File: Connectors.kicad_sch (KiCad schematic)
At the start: 12 parts, among them J10 Conn_01x12_MountingPin, J11 Conn_01x09, J15 Conn_01x12_MountingPin, J19 Conn_01x12_MountingPin, J20 Conn_01x12_MountingPin, J21 Conn_01x12_MountingPin, J25 Conn_01x03, J26 Conn_01x04, J27 Conn_01x02, J5 Conn_01x12_MountingPin, J6 Conn_01x12_MountingPin, J8 Conn_01x12_MountingPin

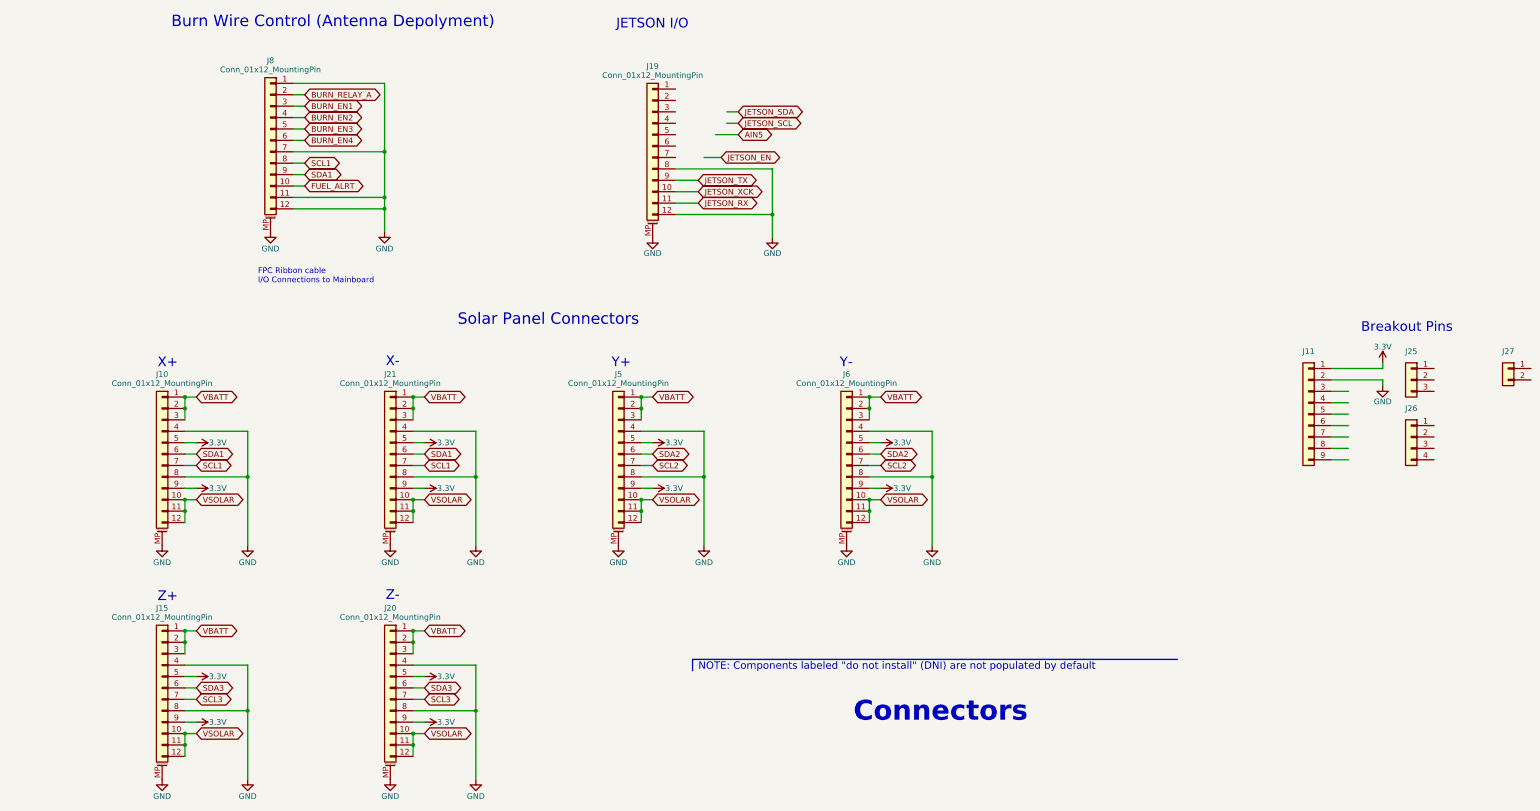
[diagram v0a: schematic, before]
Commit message: Complete layout
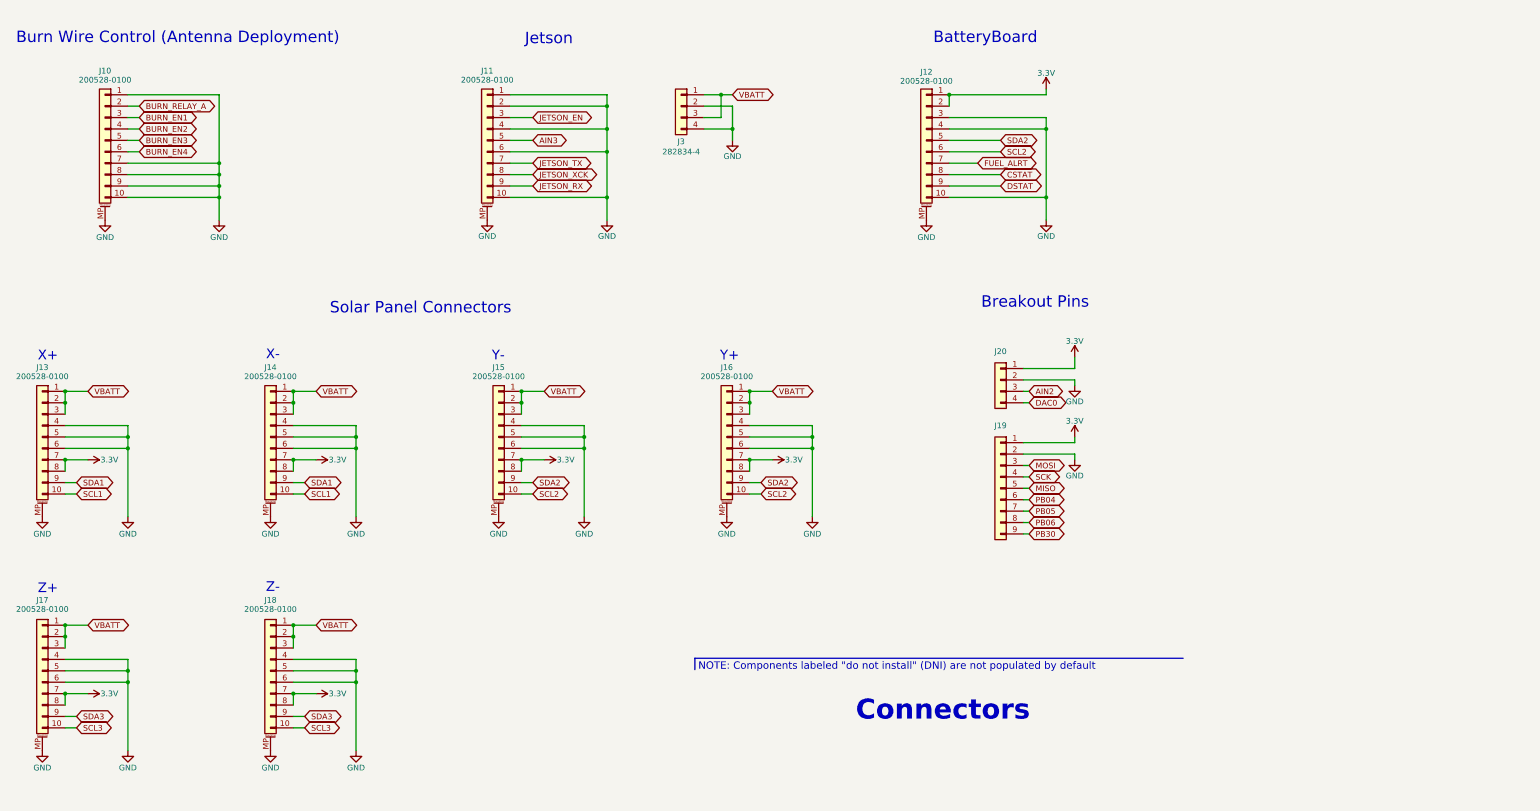
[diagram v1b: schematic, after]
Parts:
- removed J21: Conn_01x12_MountingPin, symbol Connector_Generic_MountingPin:Conn_01x12_MountingPin
- removed J25: Conn_01x03, symbol Connector_Generic:Conn_01x03
- removed J27: Conn_01x02, symbol Connector_Generic:Conn_01x02
- added J12, J14: 200528-0100, Connector_FFC-FPC:Molex_200528-0100_1x10-1MP_P1.00mm_Horizontal, symbol Connector_Generic_MountingPin:Conn_01x10_MountingPin
- added J3: 282834-4, mainboard:TE_282834-4, symbol Connector_Generic:Conn_01x04
- J10: renamed from J8; value Conn_01x12_MountingPin -> 200528-0100; footprint (none) -> Connector_FFC-FPC:Molex_200528-0100_1x10-1MP_P1.00mm_Horizontal; symbol Connector_Generic_MountingPin:Conn_01x12_MountingPin -> Connector_Generic_MountingPin:Conn_01x10_MountingPin
- J11: renamed from J19; value Conn_01x12_MountingPin -> 200528-0100; footprint (none) -> Connector_FFC-FPC:Molex_200528-0100_1x10-1MP_P1.00mm_Horizontal; symbol Connector_Generic_MountingPin:Conn_01x12_MountingPin -> Connector_Generic_MountingPin:Conn_01x10_MountingPin
- J13: renamed from J10; value Conn_01x12_MountingPin -> 200528-0100; footprint (none) -> Connector_FFC-FPC:Molex_200528-0100_1x10-1MP_P1.00mm_Horizontal; symbol Connector_Generic_MountingPin:Conn_01x12_MountingPin -> Connector_Generic_MountingPin:Conn_01x10_MountingPin
- J15: renamed from J5; value Conn_01x12_MountingPin -> 200528-0100; footprint (none) -> Connector_FFC-FPC:Molex_200528-0100_1x10-1MP_P1.00mm_Horizontal; symbol Connector_Generic_MountingPin:Conn_01x12_MountingPin -> Connector_Generic_MountingPin:Conn_01x10_MountingPin
- J16: renamed from J6; value Conn_01x12_MountingPin -> 200528-0100; footprint (none) -> Connector_FFC-FPC:Molex_200528-0100_1x10-1MP_P1.00mm_Horizontal; symbol Connector_Generic_MountingPin:Conn_01x12_MountingPin -> Connector_Generic_MountingPin:Conn_01x10_MountingPin
- J17: renamed from J15; value Conn_01x12_MountingPin -> 200528-0100; footprint (none) -> Connector_FFC-FPC:Molex_200528-0100_1x10-1MP_P1.00mm_Horizontal; symbol Connector_Generic_MountingPin:Conn_01x12_MountingPin -> Connector_Generic_MountingPin:Conn_01x10_MountingPin
- J18: renamed from J20; value Conn_01x12_MountingPin -> 200528-0100; footprint (none) -> Connector_FFC-FPC:Molex_200528-0100_1x10-1MP_P1.00mm_Horizontal; symbol Connector_Generic_MountingPin:Conn_01x12_MountingPin -> Connector_Generic_MountingPin:Conn_01x10_MountingPin
- J19: renamed from J11; footprint (none) -> Connector_PinHeader_2.54mm:PinHeader_1x09_P2.54mm_Vertical
- J20: renamed from J26; footprint (none) -> Connector_PinHeader_2.54mm:PinHeader_1x04_P2.54mm_Vertical
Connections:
- net 3.3V: now also J13.7 (Pin_7), J13.8 (Pin_8), J15.7 (Pin_7), J15.8 (Pin_8), J16.7 (Pin_7), J16.8 (Pin_8), J17.7 (Pin_7), J17.8 (Pin_8), J18.7 (Pin_7), J18.8 (Pin_8), J20.1 (Pin_1), J12.1 (Pin_1), J12.2 (Pin_2), J14.7 (Pin_7), J14.8 (Pin_8); no longer J13.5 (Pin_5), J13.9 (Pin_9), J15.5 (Pin_5), J15.9 (Pin_9), J16.5 (Pin_5), J16.9 (Pin_9), J17.5 (Pin_5), J17.9 (Pin_9), J18.5 (Pin_5), J18.9 (Pin_9)
- net FUEL_ALRT: now also J12.7 (Pin_7); no longer J10.10 (Pin_10)
- net GND: now also J10.10 (Pin_10), J10.8 (Pin_8), J10.9 (Pin_9), J11.1 (Pin_1), J11.10 (Pin_10), J11.2 (Pin_2), J11.4 (Pin_4), J11.6 (Pin_6), J13.5 (Pin_5), J13.6 (Pin_6), J15.5 (Pin_5), J15.6 (Pin_6), J16.5 (Pin_5), J16.6 (Pin_6), J17.5 (Pin_5), J17.6 (Pin_6), J18.5 (Pin_5), J18.6 (Pin_6), J20.2 (Pin_2), J12.10 (Pin_10), J12.3 (Pin_3), J12.4 (Pin_4), J12.MP (MountPin), J14.4 (Pin_4), J14.5 (Pin_5), J14.6 (Pin_6), J14.MP (MountPin), J3.2 (Pin_2), J3.4 (Pin_4); no longer J10.11 (Pin_11), J10.12 (Pin_12), J11.12 (Pin_12), J11.8 (Pin_8), J13.8 (Pin_8), J15.8 (Pin_8), J16.8 (Pin_8), J17.8 (Pin_8), J18.8 (Pin_8)
- net JETSON_EN: now also J11.3 (Pin_3)
- net JETSON_RX: now also J11.9 (Pin_9); no longer J11.11 (Pin_11)
- net JETSON_TX: now also J11.7 (Pin_7); no longer J11.9 (Pin_9)
- net JETSON_XCK: now also J11.8 (Pin_8); no longer J11.10 (Pin_10)
- net SCL1: now also J13.10 (Pin_10), J14.10 (Pin_10); no longer J10.8 (Pin_8), J13.7 (Pin_7)
- net SCL2: now also J15.10 (Pin_10), J16.10 (Pin_10), J12.6 (Pin_6); no longer J15.7 (Pin_7), J16.7 (Pin_7)
- net SCL3: now also J17.10 (Pin_10), J18.10 (Pin_10); no longer J17.7 (Pin_7), J18.7 (Pin_7)
- net SDA1: now also J13.9 (Pin_9), J14.9 (Pin_9); no longer J10.9 (Pin_9), J13.6 (Pin_6)
- net SDA2: now also J15.9 (Pin_9), J16.9 (Pin_9), J12.5 (Pin_5); no longer J15.6 (Pin_6), J16.6 (Pin_6)
- net SDA3: now also J17.9 (Pin_9), J18.9 (Pin_9); no longer J17.6 (Pin_6), J18.6 (Pin_6)
- net VBATT: now also J14.1 (Pin_1), J14.2 (Pin_2), J14.3 (Pin_3), J3.1 (Pin_1), J3.3 (Pin_3)
- net AIN2: now reaches J20.3 (Pin_3)
- net DAC0: now reaches J20.4 (Pin_4)
- net AIN3: now reaches J11.5 (Pin_5)
- net MOSI: now reaches J19.3 (Pin_3)
- net SCK: now reaches J19.4 (Pin_4)
- net MISO: now reaches J19.5 (Pin_5)
- net PB04: now reaches J19.6 (Pin_6)
- net PB05: now reaches J19.7 (Pin_7)
- net PB06: now reaches J19.8 (Pin_8)
- net PB30: now reaches J19.9 (Pin_9)
- removed net VSOLAR: J13.10 (Pin_10), J13.11 (Pin_11), J13.12 (Pin_12), J15.10 (Pin_10), J15.11 (Pin_11), J15.12 (Pin_12), J16.10 (Pin_10), J16.11 (Pin_11), J16.12 (Pin_12), J17.10 (Pin_10), J17.11 (Pin_11), J17.12 (Pin_12), J18.10 (Pin_10), J18.11 (Pin_11), J18.12 (Pin_12)
- new net CSTAT: J12.8 (Pin_8)
- new net DSTAT: J12.9 (Pin_9)
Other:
- note added: "BatteryBoard"
- note added: "Burn Wire Control (Antenna Deployment)"
- note added: "Jetson"
- note removed: "Burn Wire Control (Antenna Depolyment)"
- note removed: "FPC Ribbon cable I/O Connections to Mainboard"
- note removed: "JETSON I/O"
- moved on the sheet: J19, J20

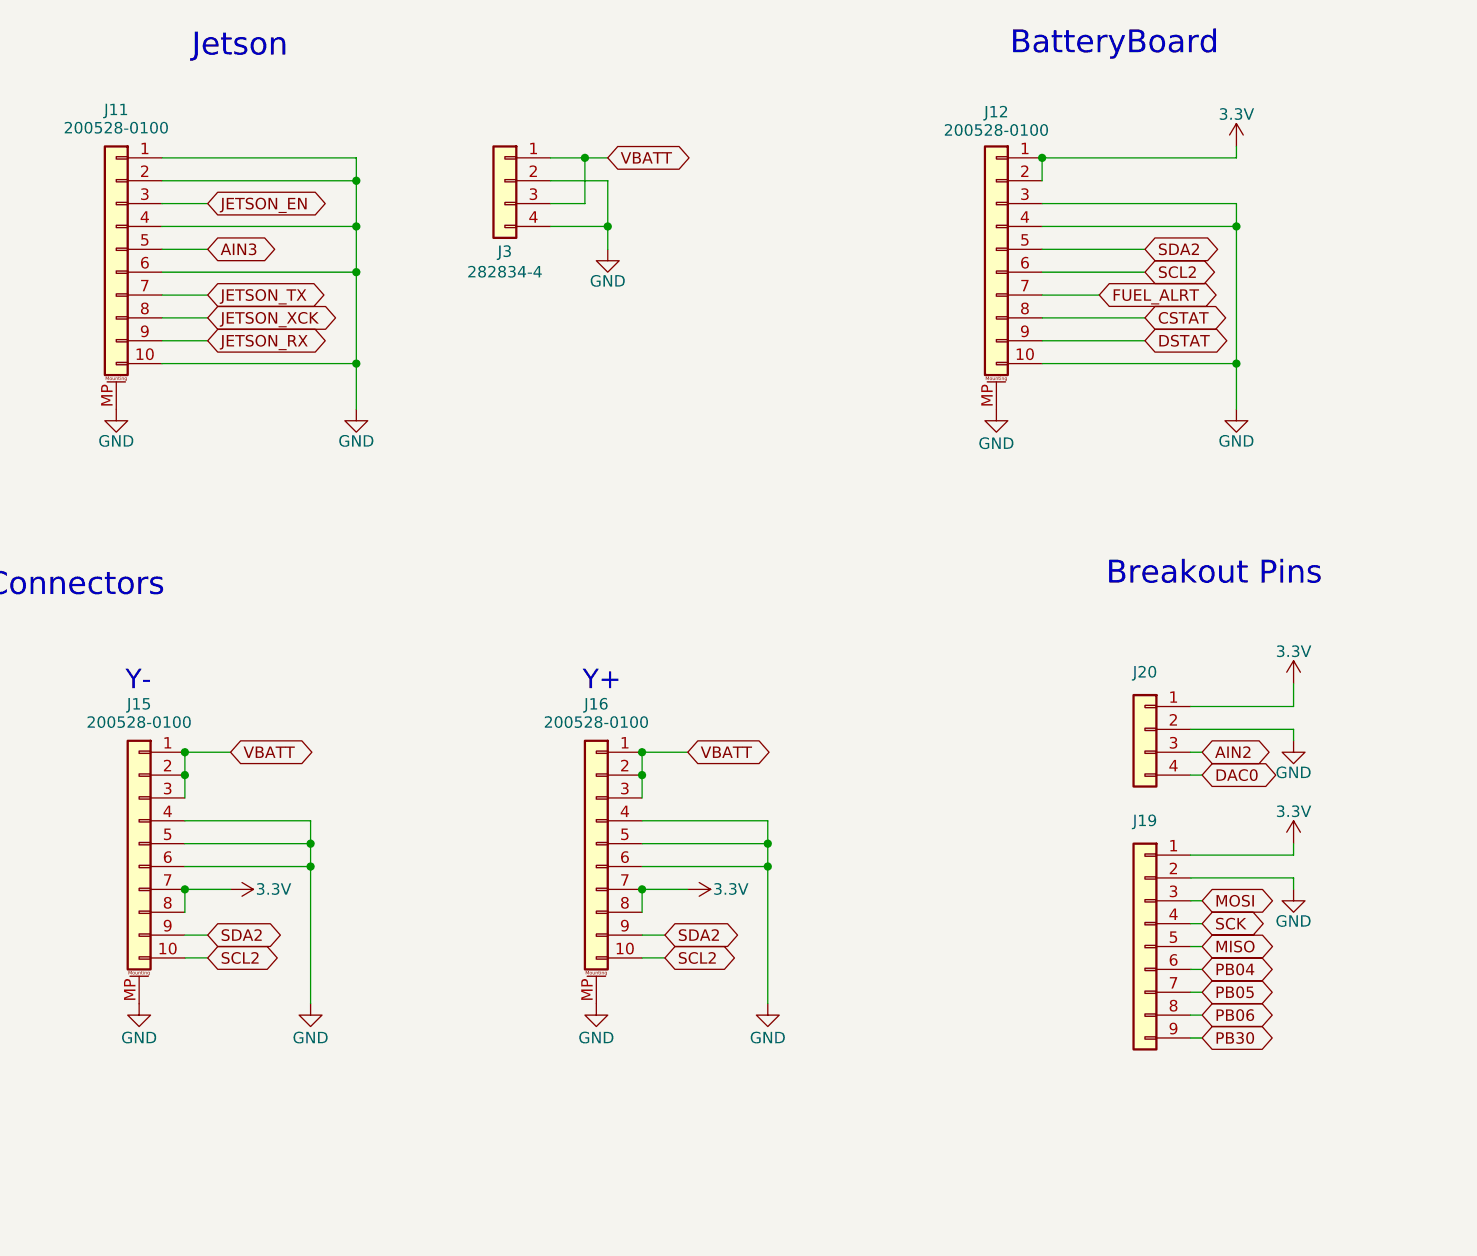
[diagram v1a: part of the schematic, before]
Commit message: v1 Final
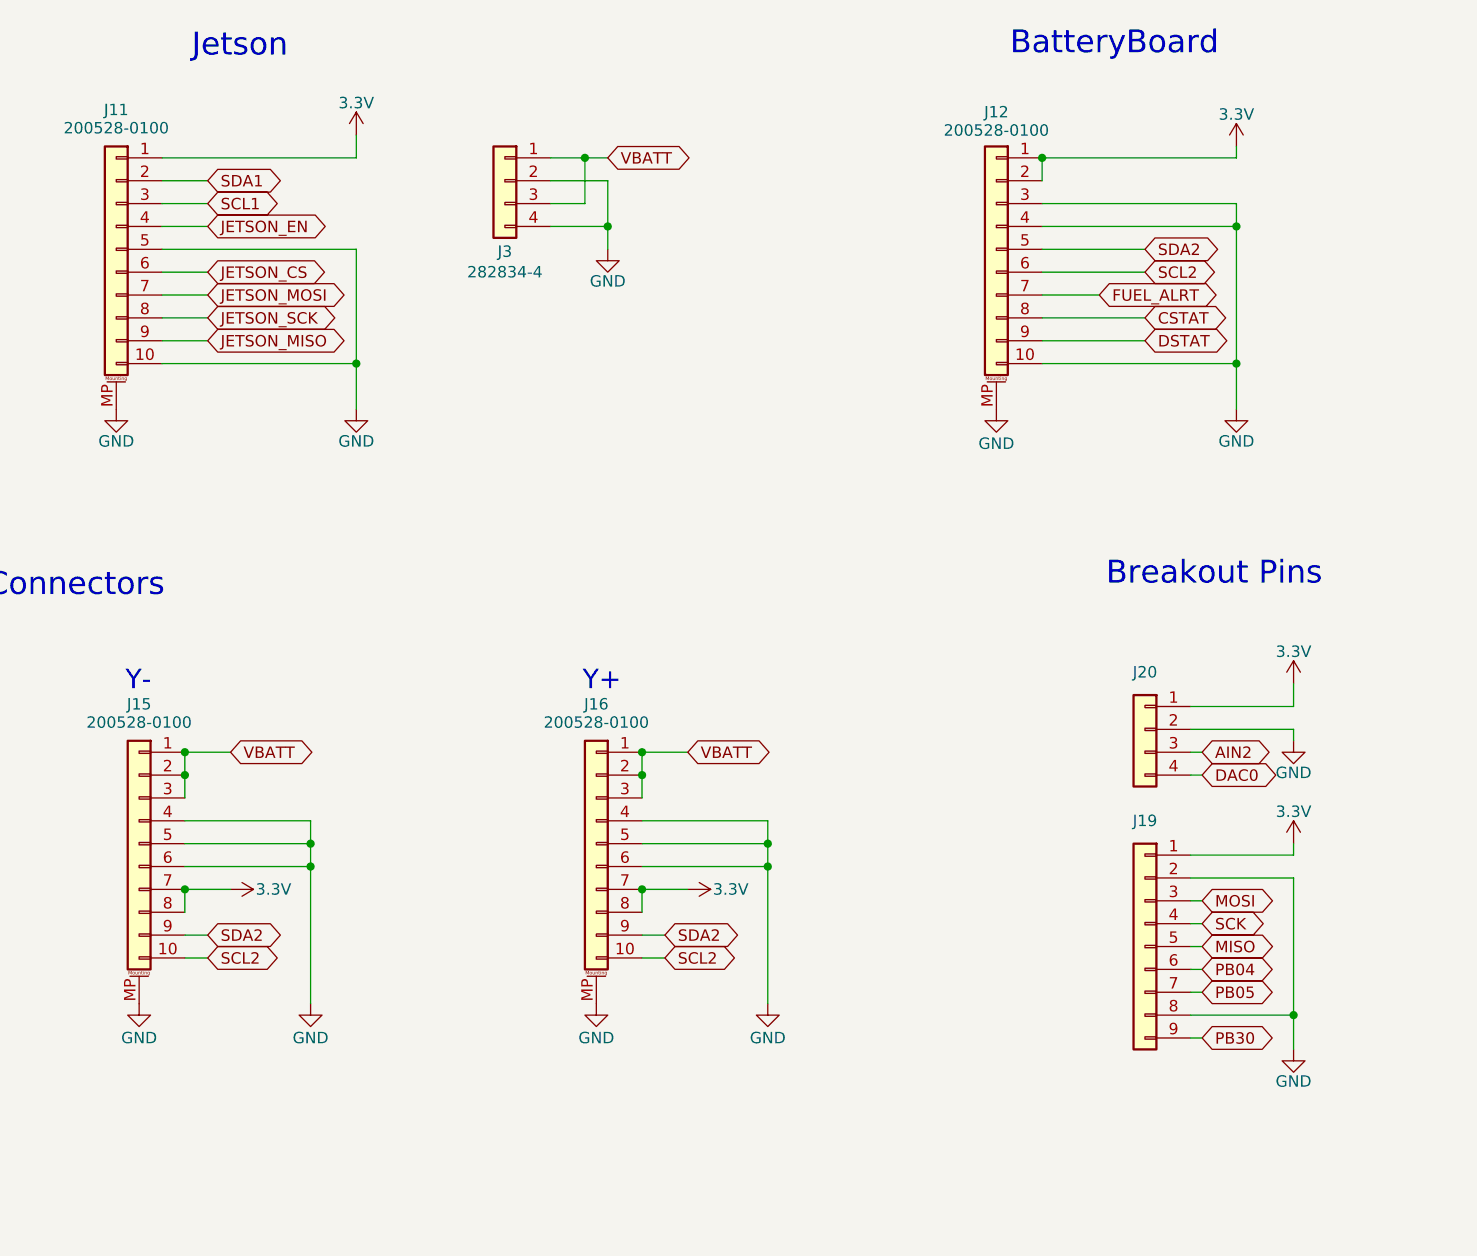
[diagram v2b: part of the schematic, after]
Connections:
- net AIN3 is gone; now on net GND: J11.5 (Pin_5)
- net PB06 is gone; now on net GND: J19.8 (Pin_8)
- net 3.3V: now also J11.1 (Pin_1)
- net GND: no longer J11.1 (Pin_1), J11.2 (Pin_2), J11.4 (Pin_4), J11.6 (Pin_6)
- net JETSON_EN: now also J11.4 (Pin_4); no longer J11.3 (Pin_3)
- net SCL1: now also J11.3 (Pin_3)
- net SDA1: now also J11.2 (Pin_2)
- net JETSON_RX renamed JETSON_MISO
- net JETSON_TX renamed JETSON_MOSI
- net JETSON_XCK renamed JETSON_SCK
- new net JETSON_CS: J11.6 (Pin_6)

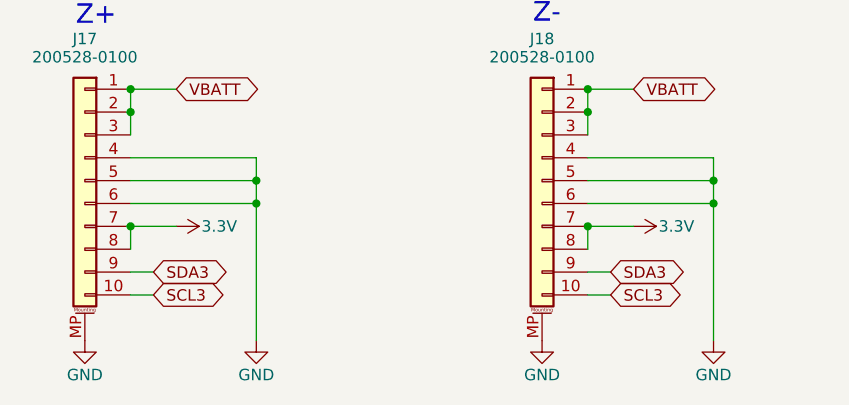
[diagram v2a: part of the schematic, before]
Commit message: Stash
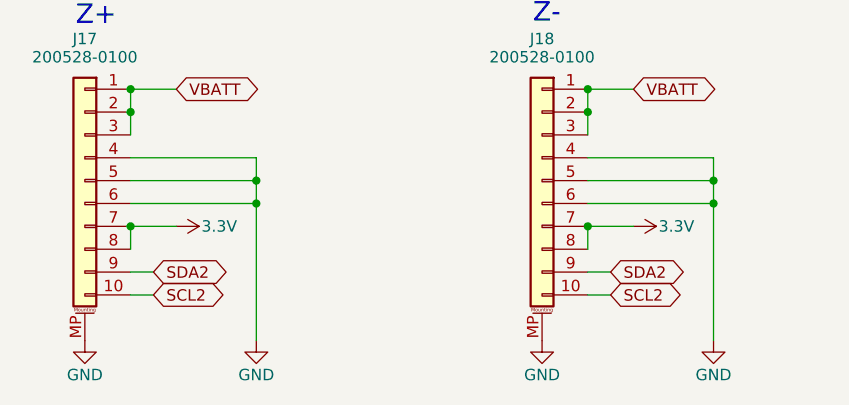
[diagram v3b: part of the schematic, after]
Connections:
- net SCL3 is gone; now on net SCL2: J17.10 (Pin_10), J18.10 (Pin_10)
- net SDA3 is gone; now on net SDA2: J17.9 (Pin_9), J18.9 (Pin_9)
